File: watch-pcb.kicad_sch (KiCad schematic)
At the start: 12 parts, among them J1 DAUGHTER

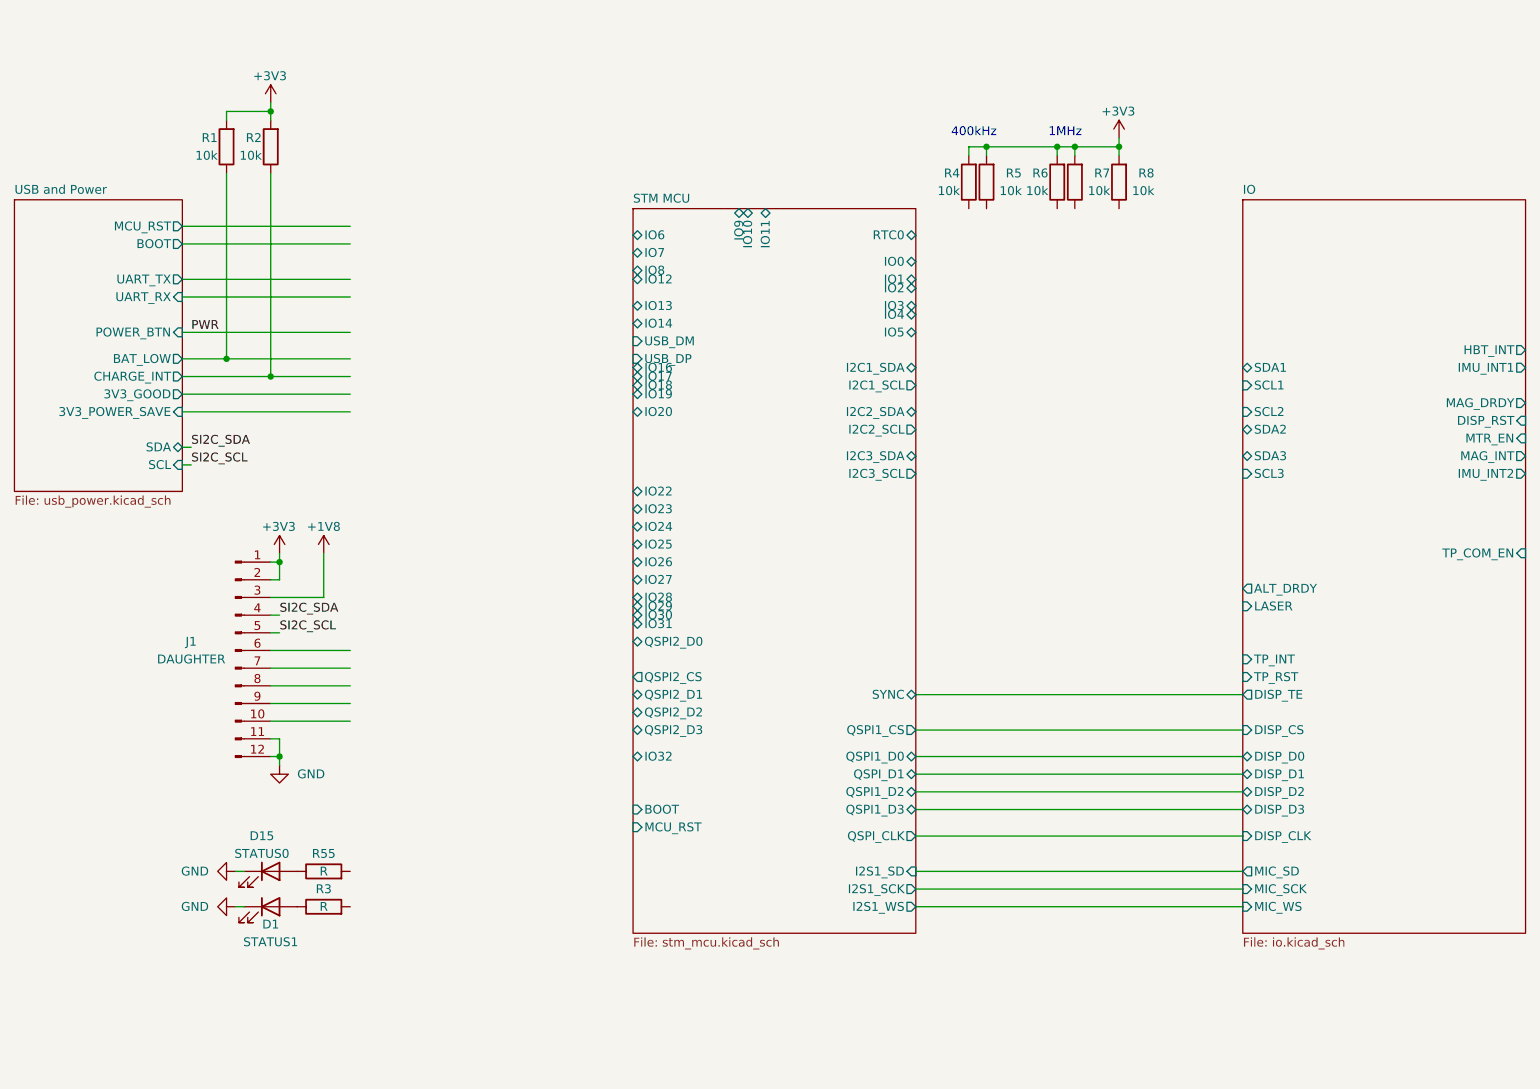
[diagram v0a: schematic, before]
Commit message: quicksaving pcb bc im gonna redo it
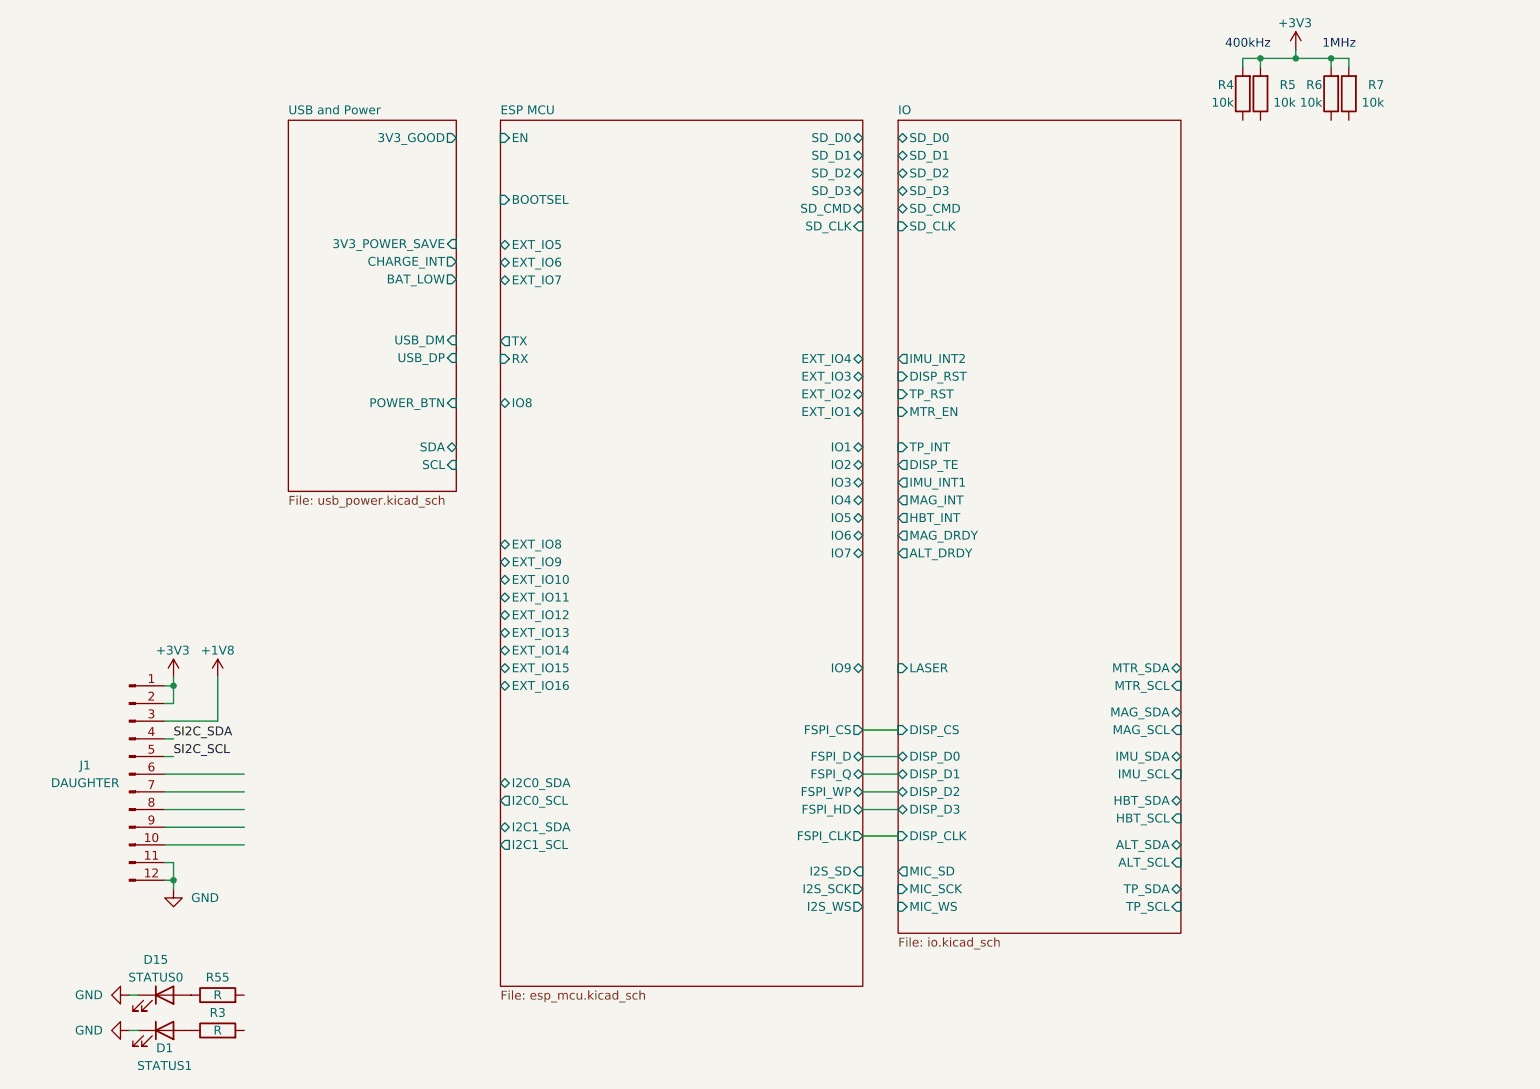
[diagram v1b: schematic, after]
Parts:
- removed R1, R2, R8: 10k, Resistor_SMD:R_0402_1005Metric, symbol Device:R
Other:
- removed sheet STM MCU
- added sheet ESP MCU (esp_mcu.kicad_sch)
- sheet IO ports: added ALT_SCL, ALT_SDA, HBT_SCL, HBT_SDA, IMU_SCL, IMU_SDA, MAG_SCL, MAG_SDA, MTR_SCL, MTR_SDA, SD_CLK, SD_CMD, SD_D0, SD_D1, SD_D2, SD_D3, TP_SCL, TP_SDA; removed SCL1, SCL2, SCL3, SDA1, SDA2, SDA3, TP_COM_EN
- sheet USB and Power ports: added USB_DM, USB_DP; removed BOOT, MCU_RST, UART_RX, UART_TX
- moved on the sheet: D1, D15, J1, R3, R4, R5, R55, R6, R7
